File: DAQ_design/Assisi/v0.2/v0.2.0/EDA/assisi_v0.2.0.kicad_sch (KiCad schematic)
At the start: 18 parts, among them J1 Screw_Terminal_01x05, Q1 BC549, Q2 IRF9540N, Q3 IRF540N, Q4 BC549, Q5 IRF540N, Q6 IRF9540N

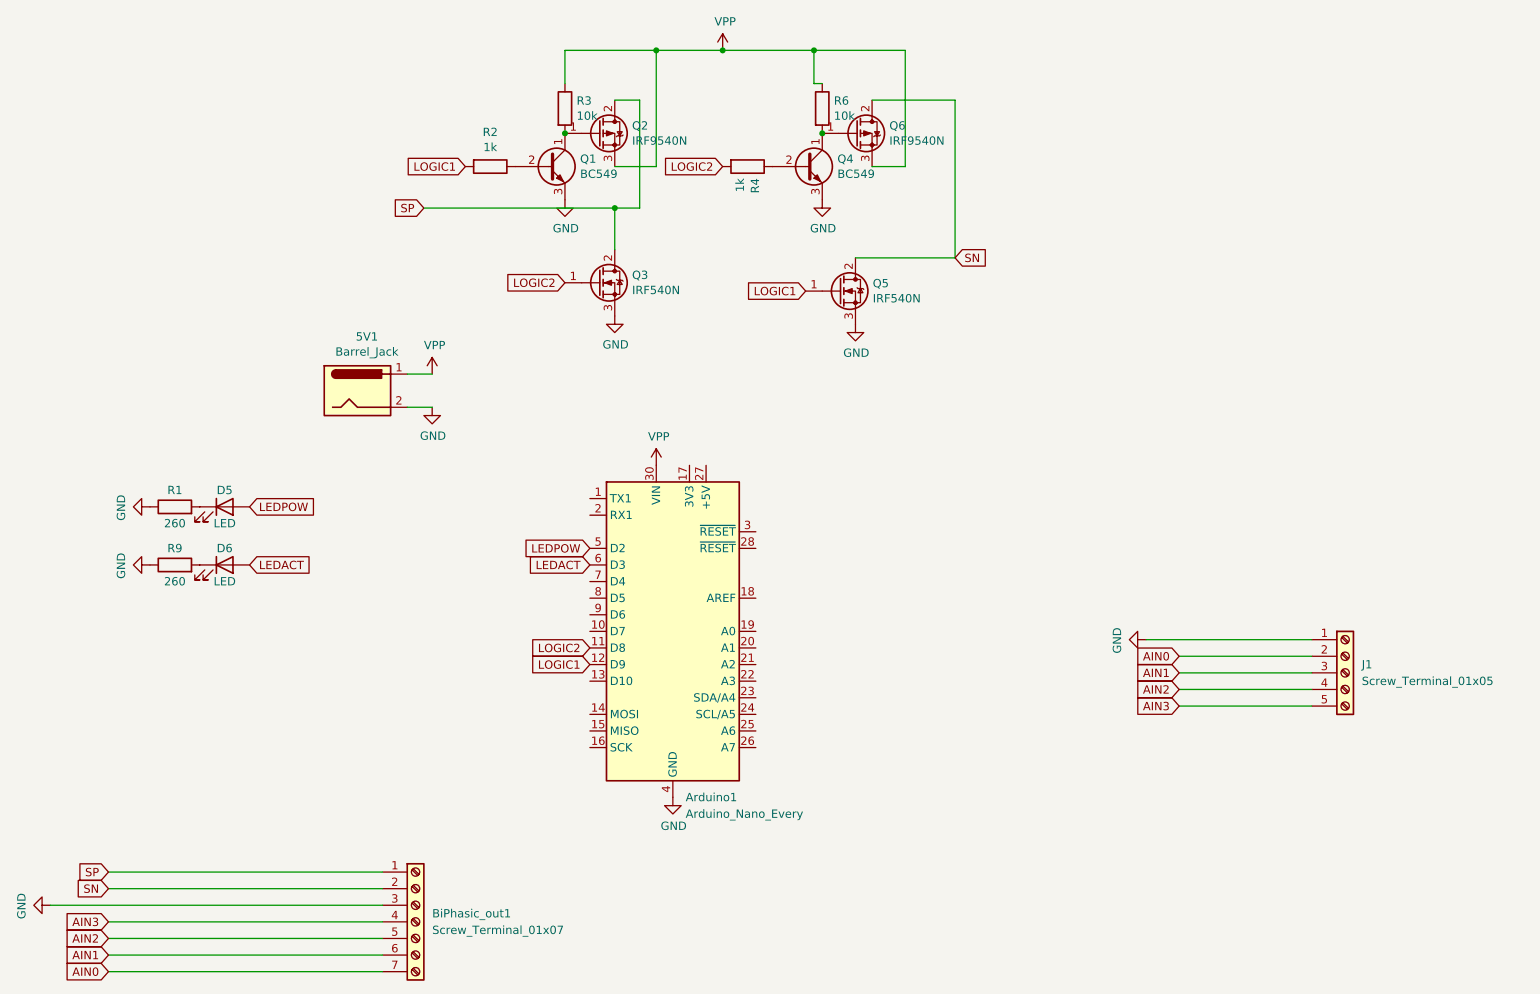
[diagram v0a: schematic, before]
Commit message: new assisi v0.2.0 pcb design
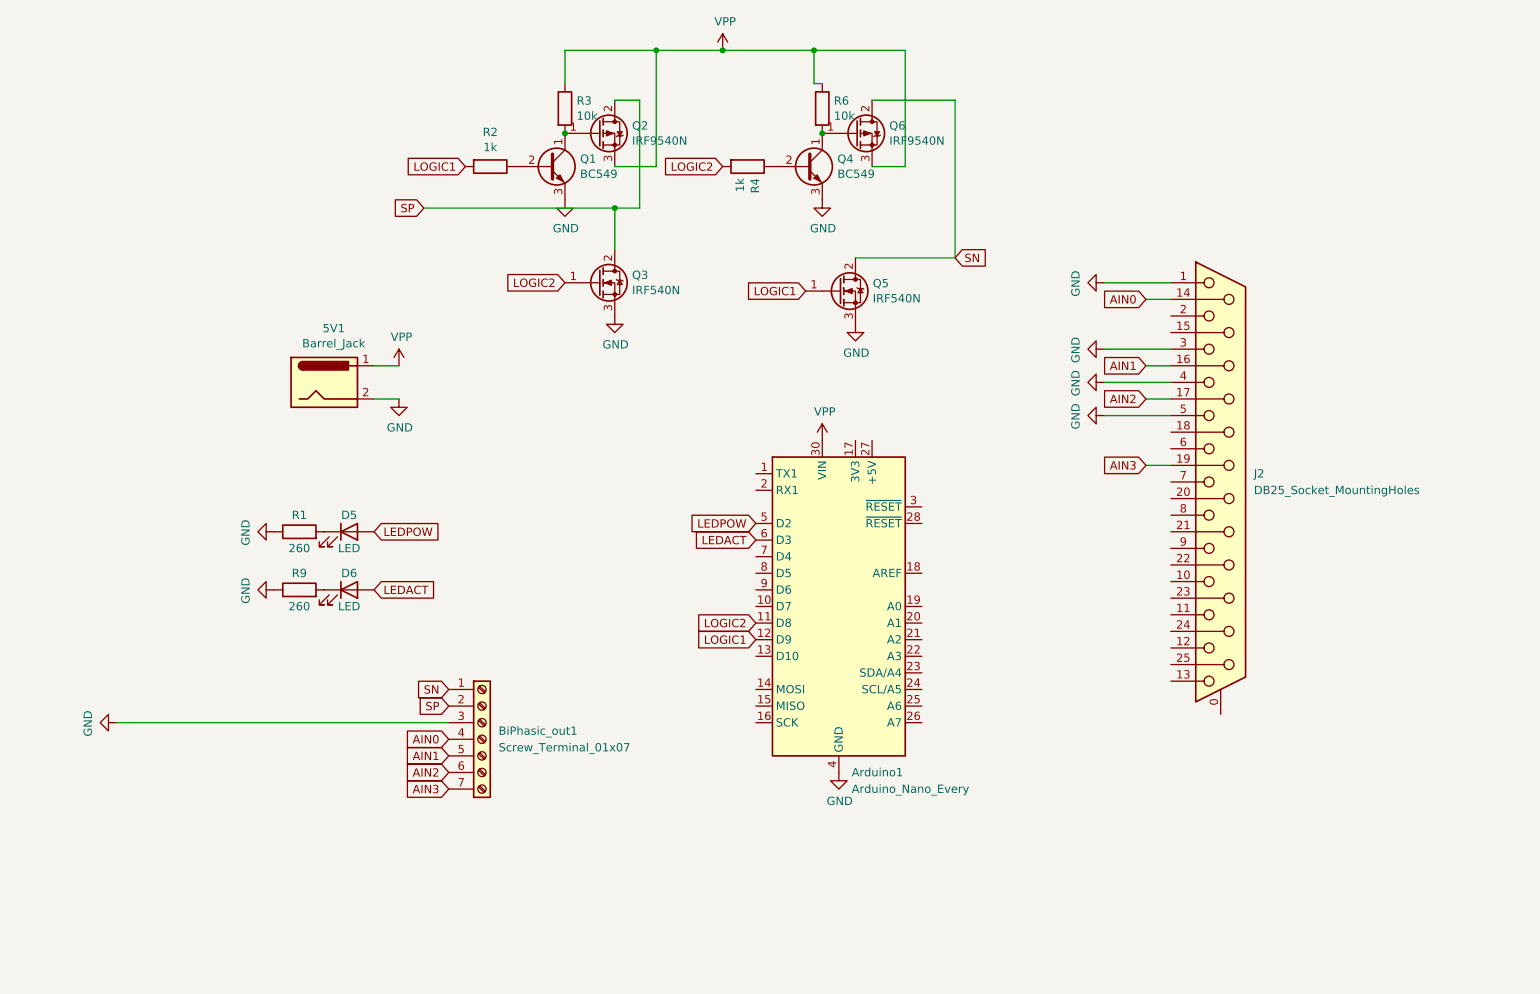
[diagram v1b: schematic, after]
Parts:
- removed J1: Screw_Terminal_01x05, symbol Connector:Screw_Terminal_01x05
- added J2: DB25_Socket_MountingHoles, Connector_Dsub:DSUB-25_Pins_Horizontal_P2.77x2.84mm_EdgePinOffset7.70mm_Housed_MountingHolesOffset9.12mm, symbol Connector:DB25_Socket_MountingHoles
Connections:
- net AIN0: now also BiPhasic_out1.4 (Pin_4), J2.14 (P14); no longer BiPhasic_out1.7 (Pin_7)
- net AIN1: now also BiPhasic_out1.5 (Pin_5), J2.16 (P16); no longer BiPhasic_out1.6 (Pin_6)
- net AIN2: now also BiPhasic_out1.6 (Pin_6), J2.17 (P17); no longer BiPhasic_out1.5 (Pin_5)
- net AIN3: now also BiPhasic_out1.7 (Pin_7), J2.19 (P19); no longer BiPhasic_out1.4 (Pin_4)
- net GND: now also J2.1, J2.3, J2.4, J2.5
- net SN: now also BiPhasic_out1.1 (Pin_1); no longer BiPhasic_out1.2 (Pin_2)
- net SP: now also BiPhasic_out1.2 (Pin_2); no longer BiPhasic_out1.1 (Pin_1)
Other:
- company: (none) -> ARTS-Lab at the University of South Carolina
- title: (none) -> Biphasic PCB: Assisi V0.2.0
- moved on the sheet: 5V1, Arduino1, BiPhasic_out1, D5, D6, R1, R9
